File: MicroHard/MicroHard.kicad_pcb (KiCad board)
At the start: 4 copper layers, 200 parts, among them IC1 IS66WVO32M8DBLL-166BLI, J1 USB_B_Micro, J2 Micro_SD_Card_Det2, J3 GPIO_header, J4 MCU_Debug, J5 Controller Connector, J6 FPGA_GPIO_header, J7 FPGA_DEBUG, J8 L77HDE15SD1CH4FVGA, SW1 KMR221NGLFS, SW2 KMR221NGLFS, SW3 KMR221NGLFS, SW4 KMR221NGLFS, U1 TPS54325, U2 TPS54294, U3 EFM32GG842F1024, U4 XC7A100T-FTG256, U5 MAX6955 Display Driver, U6 SN74ALVC245PWR, U7 SN74ALVC245PWR, U8 MT25QL256ABA8ESF-0SIT, Y1 48MHz, Y2 CB3-3C-20M000000

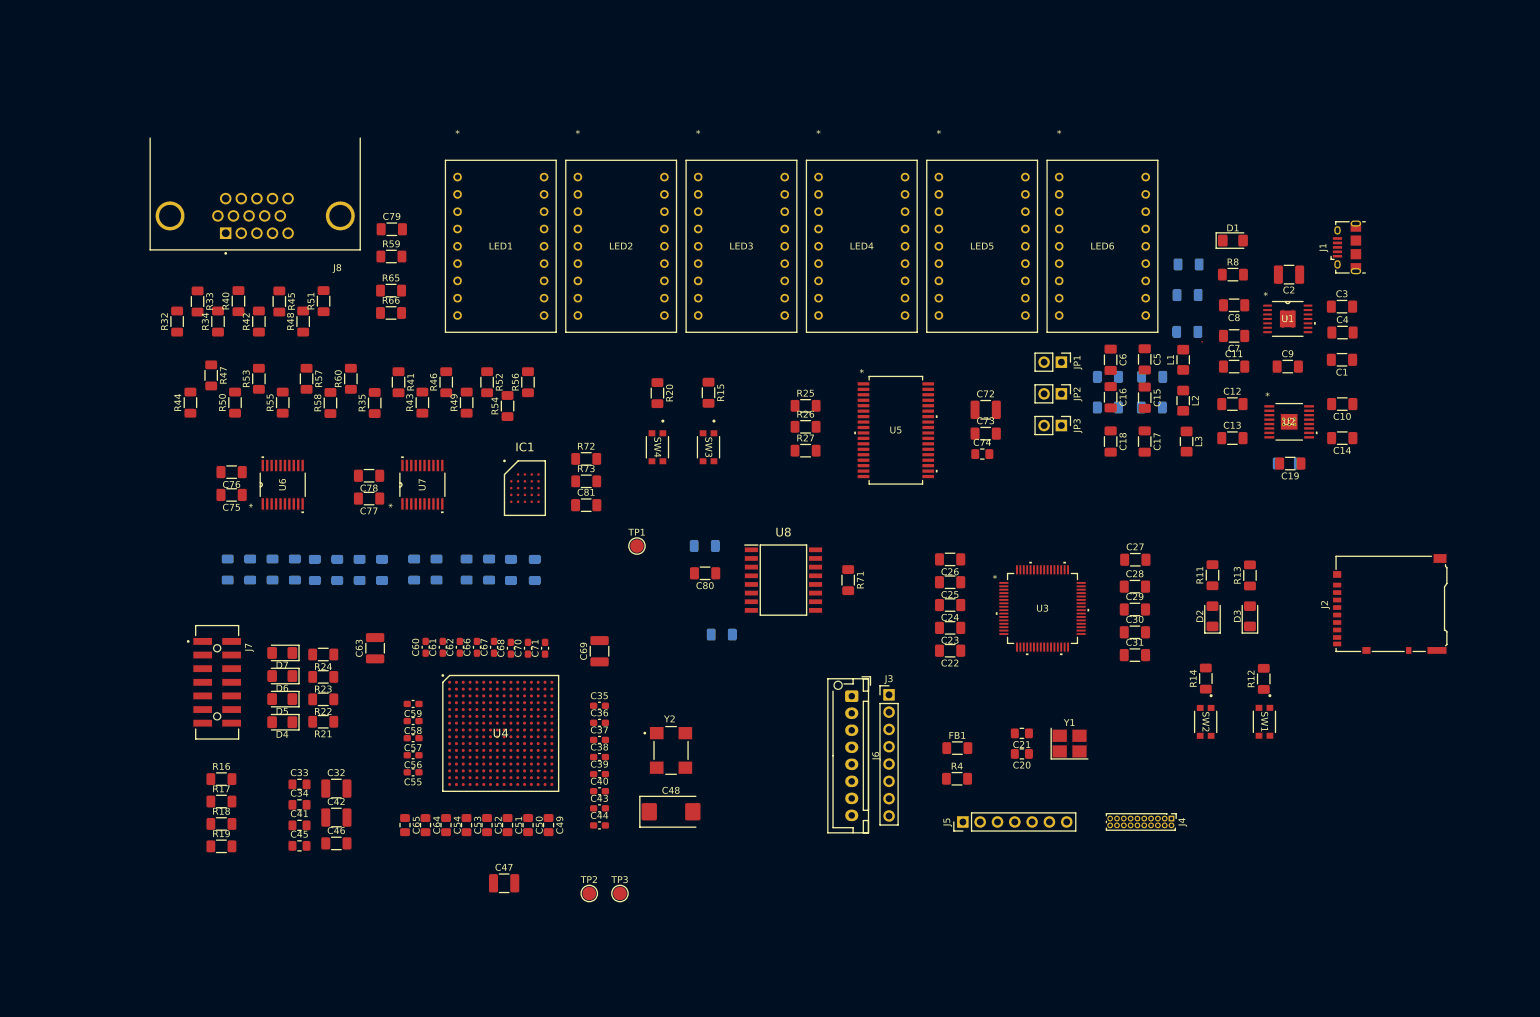
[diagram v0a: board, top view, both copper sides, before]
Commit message: VGA and Display layout
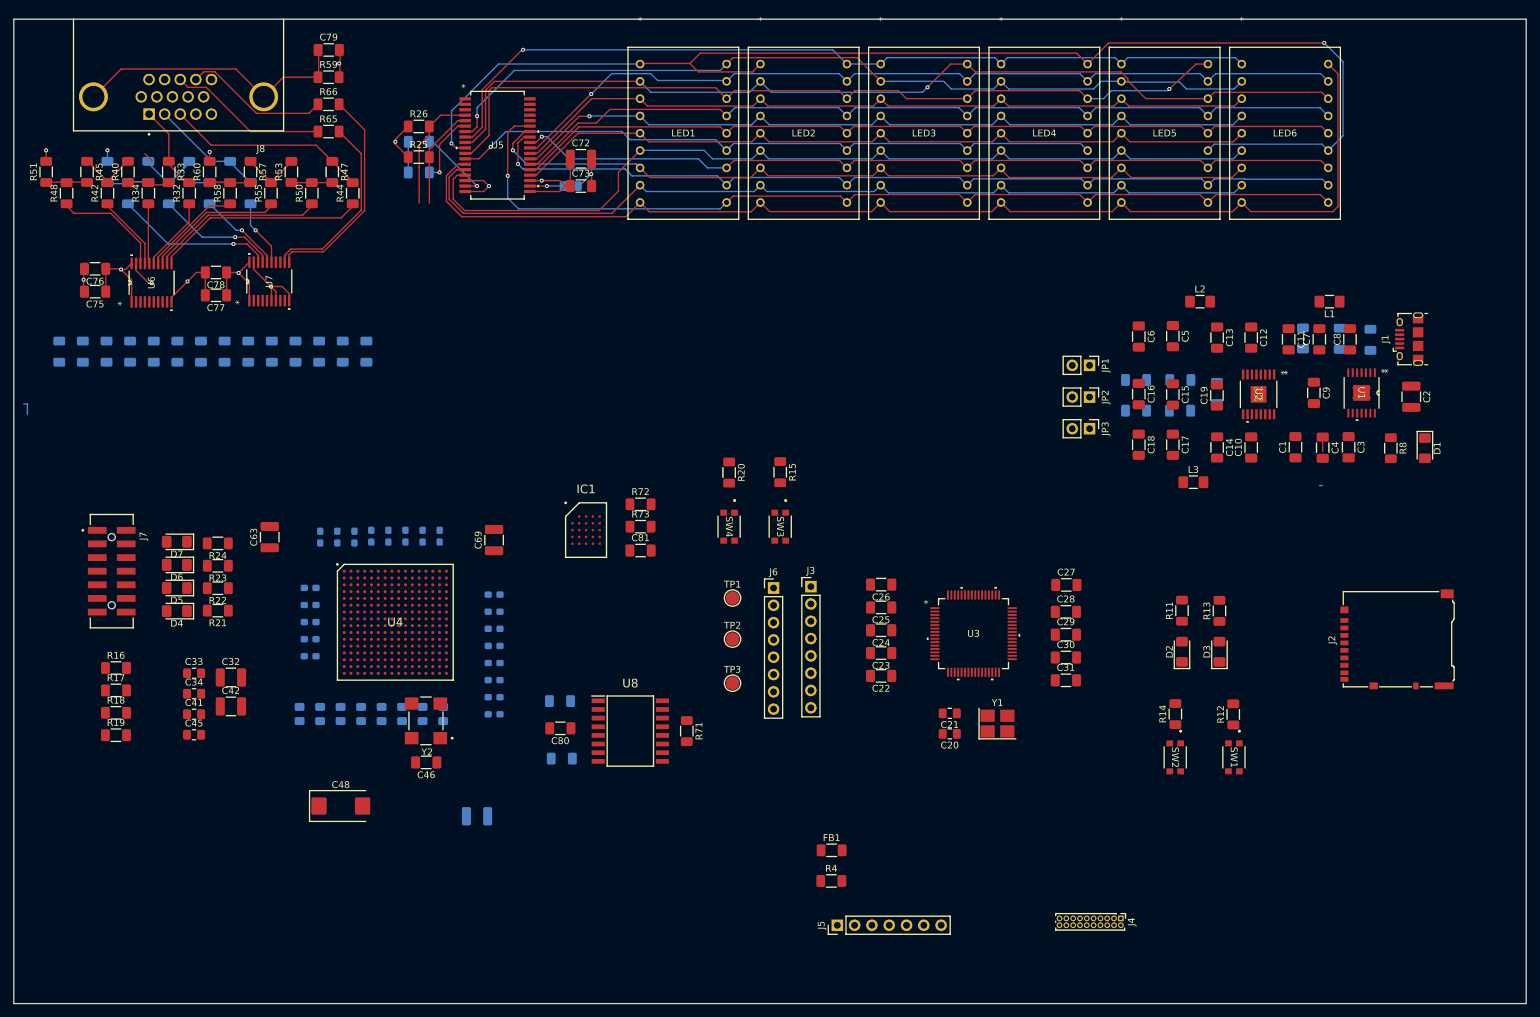
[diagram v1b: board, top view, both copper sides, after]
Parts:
- added R74: 12k, Resistor_SMD:R_1206_3216Metric_Pad1.30x1.75mm_HandSolder, B.Cu at (97.5, 51.5)
- C35, C36, C37, C38, C39, C40, C43, C44, C47, C49, C50, C51, C52, C53, C54, C55, C56, C57, C58, C59, C60, C61, C62, C64, C65, C66, C67, C68, C70, C71, C74, R35, R41, R43, R46, R49, R52, R54, R56: moved to B.Cu
- J6: footprint Connector_JST:JST_XH_B8B-XH-AM_1x08_P2.50mm_Vertical -> Connector_PinHeader_2.54mm:PinHeader_1x08_P2.54mm_Vertical
- R27: value 112k -> 100k; moved to B.Cu
- R8: value 68 -> 330
- moved R27 72.7 mm to (97.5, 47.0), turned to 180 degrees
- moved C74 72.1 mm to (119.8, 53.5)
- moved U5 71.9 mm to (109.0, 47.5)
- moved R26 71.9 mm to (97.5, 44.8)
- moved C72 69.9 mm to (121.2, 49.5)
- moved C73 69.6 mm to (121.2, 53.5)
- moved R56 69.0 mm to (51.8, 51.4)
- moved R25 67.5 mm to (97.5, 49.2)
- moved R54 63.9 mm to (54.8, 54.5)
- moved R52 58.5 mm to (57.8, 51.4)
- moved R49 53.4 mm to (60.8, 54.5)
- moved R46 48.7 mm to (63.8, 51.4)
- moved C48 48.5 mm to (86.0, 144.5)
- moved R51 44.9 mm to (42.7, 51.4)
- moved R43 43.8 mm to (66.8, 54.5)
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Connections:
- R27 pad 2: GND -> Net-(R27-Pad2)
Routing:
- net DD_O3: track 0.00 -> 188.2 mm, vias 0 -> 2
- net DD_O6: track 0.00 -> 167.8 mm
- net DD_O2: track 0.00 -> 141.1 mm, vias 0 -> 1
- net DD_O18: track 0.00 -> 139.4 mm, vias 0 -> 1
- net DD_O8: track 0.00 -> 131.7 mm
- net DD_O16: track 0.00 -> 129.6 mm, vias 0 -> 1
- net DD_O7: track 0.00 -> 129.3 mm
- net DD_O14: track 0.00 -> 126.9 mm, vias 0 -> 1
- net DD_O11: track 0.00 -> 125.9 mm
- net DD_O1: track 0.00 -> 125.8 mm, vias 0 -> 1
- net DD_O0: track 0.00 -> 125.4 mm, vias 0 -> 1
- net DD_O10: track 0.00 -> 124.3 mm
- net DD_O15: track 0.00 -> 123.9 mm, vias 0 -> 1
- net DD_O4: track 0.00 -> 122.7 mm, vias 0 -> 1
- net DD_O17: track 0.00 -> 117.9 mm, vias 0 -> 1
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- added copper zone on In2.Cu, net +3.3V
- added copper zone on In1.Cu, net GND
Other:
- board outline added: 222 x 144.5 mm
